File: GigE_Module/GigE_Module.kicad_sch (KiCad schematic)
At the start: 25 parts, among them J1 Conn_01x10_Socket, J2 Conn_01x10_Socket, J3 RJ45_Amphenol_RJMG1BD3B8K1ANR, U4 ENC28J60x-SS, Y1 25MHz

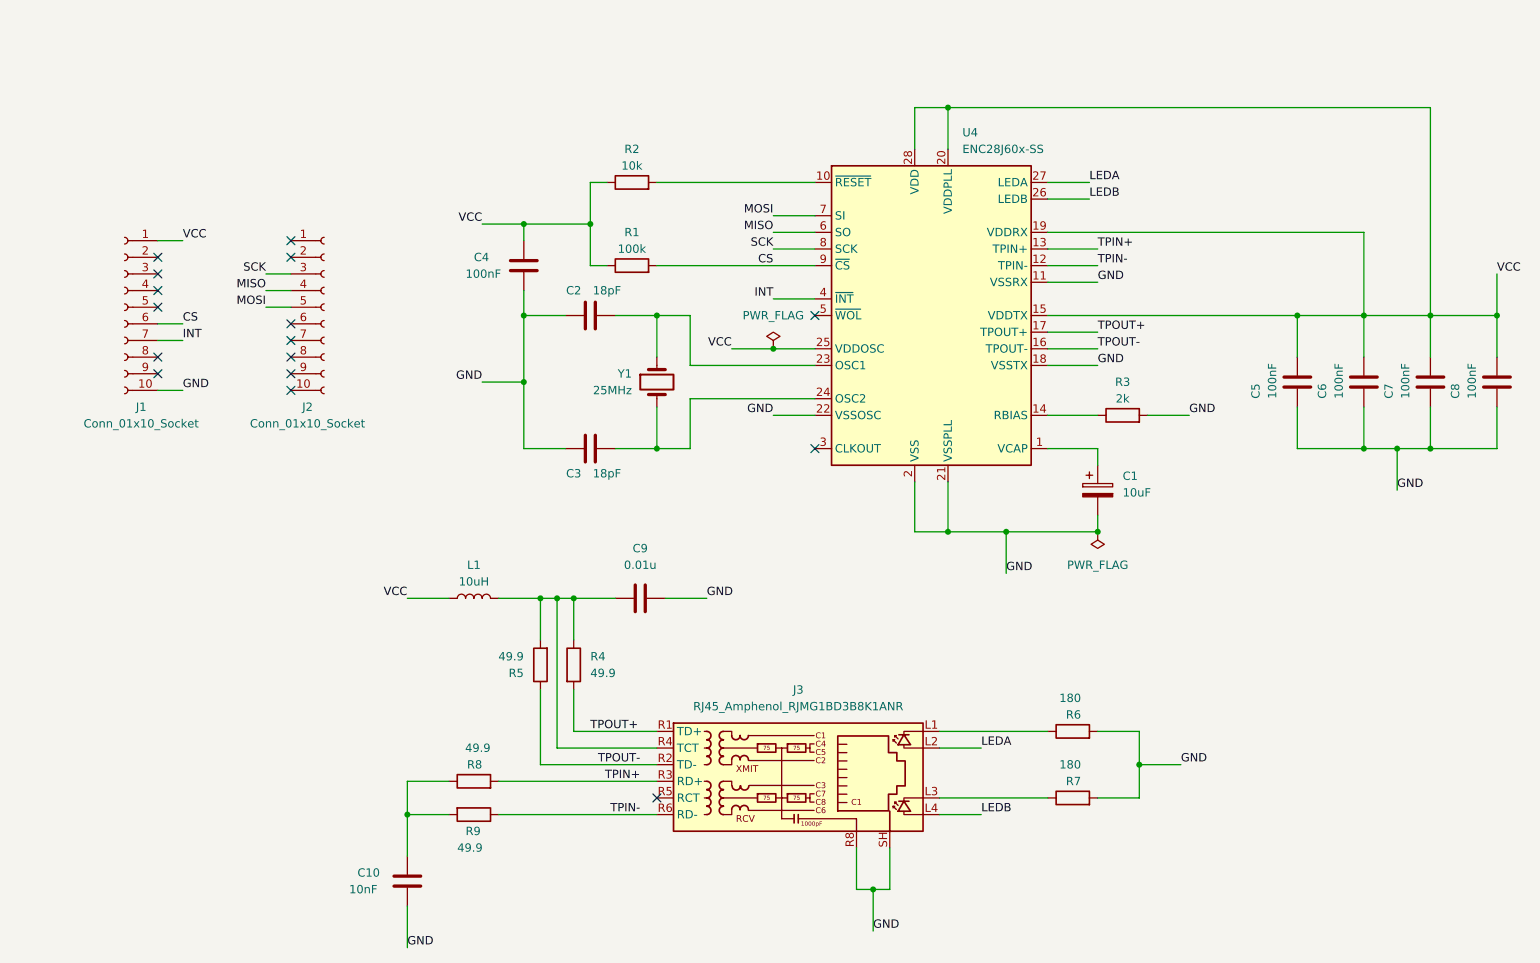
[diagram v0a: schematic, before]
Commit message: Finishing GigE PCB design
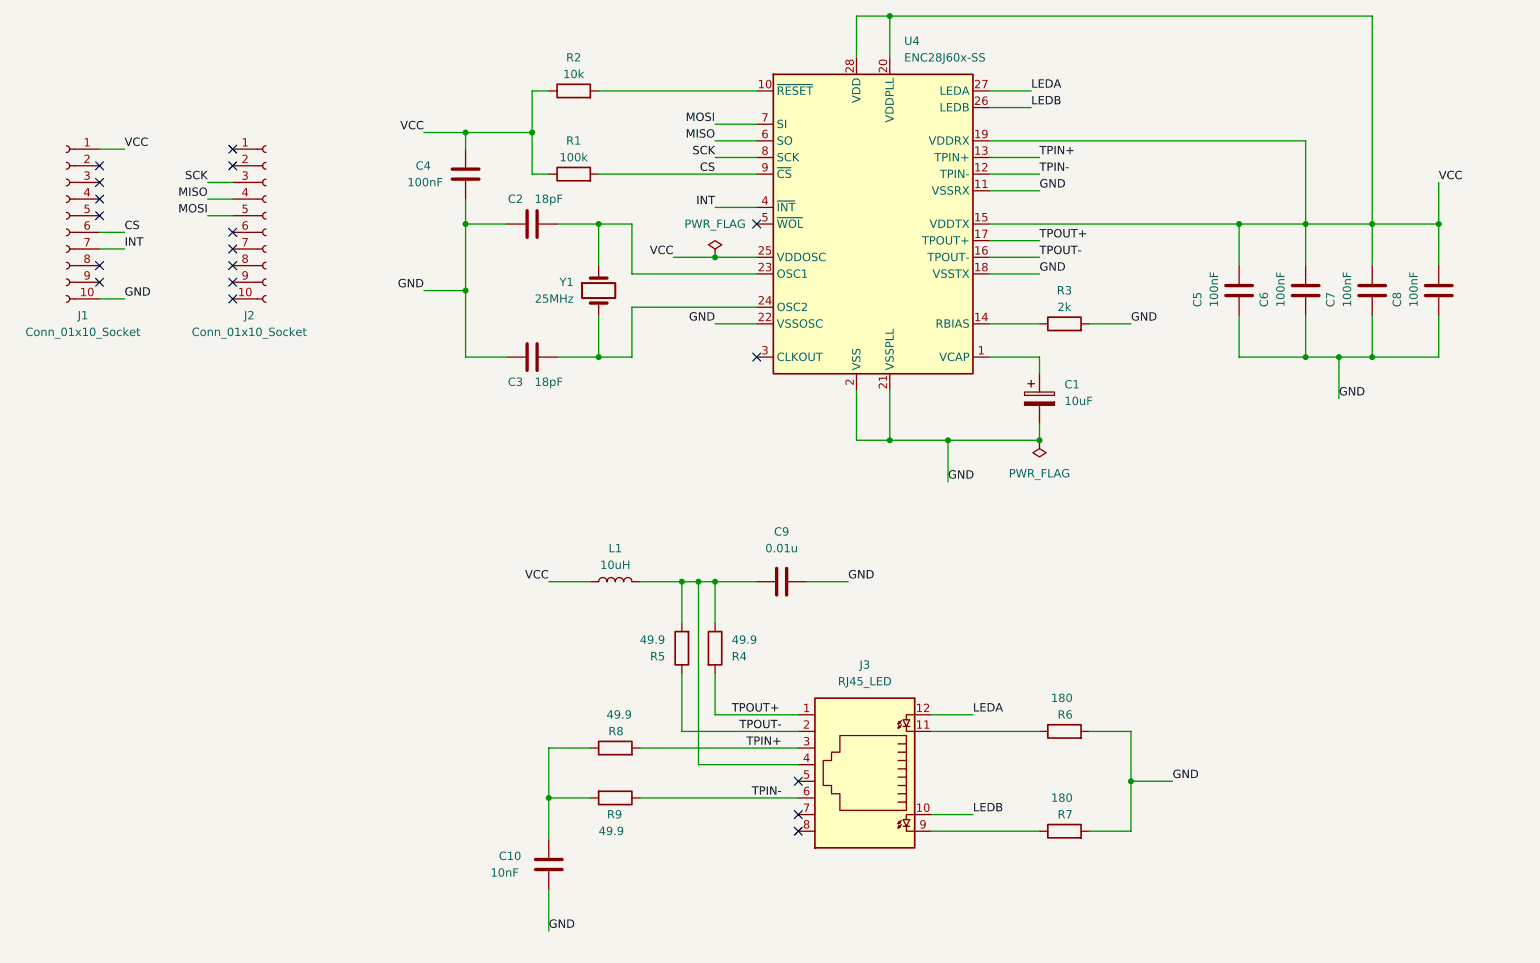
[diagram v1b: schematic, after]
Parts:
- removed J3: RJ45_Amphenol_RJMG1BD3B8K1ANR, Connector_RJ:RJ45_Amphenol_RJHSE538X, symbol Connector:RJ45_Amphenol_RJMG1BD3B8K1ANR
- added J3: RJ45_LED, Connector_RJ:RJ45_Amphenol_RJHSE538X, symbol Connector:RJ45_LED
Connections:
- net LEDA: now also J3.12
- net LEDB: now also J3.10
- net TPIN+: now also J3.3
- net TPIN-: now also J3.6
- net TPOUT+: now also J3.1
- net TPOUT-: now also J3.2
- net at C9.1, L1.2, R4.1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: now also J3.4
- net at R6.1: now also J3.11
- net at R7.1: now also J3.9
- no-connect marks 16 -> 18
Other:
- moved on the sheet: C1, C2, C3, C4, C5, C6, C7, C8, J1, J2, R1, R2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
